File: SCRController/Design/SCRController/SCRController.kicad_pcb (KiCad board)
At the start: 2 copper layers, 76.9 x 73 mm, 43 parts, among them J1 VALT, J2 SAL_TRIAC, Q1 2N2907A, Q2 2N2222A, Q3 2N2222A, Q4 2N2907A, U1 TL084, U2 TL084, U3 LM7815_TO220, U4 LM7915_TO220, U5 MOC3011M

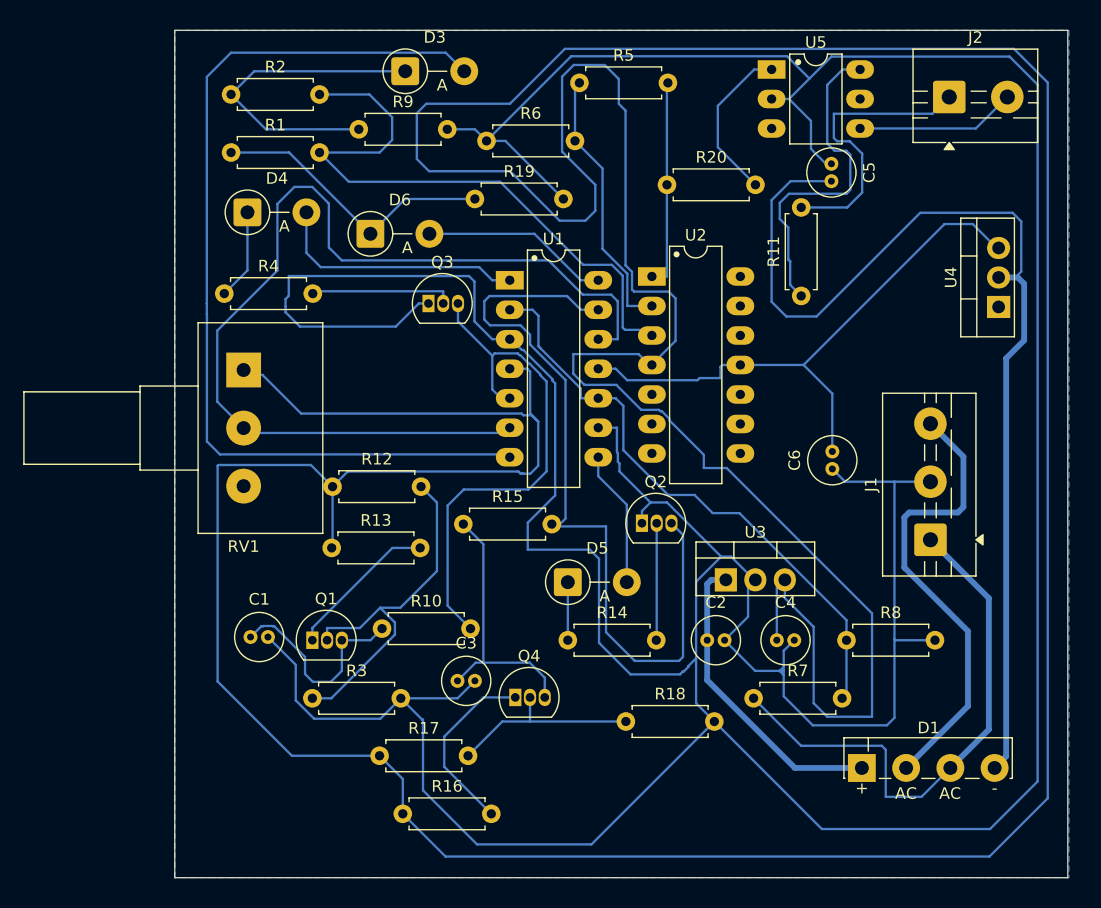
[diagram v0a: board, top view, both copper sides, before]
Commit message: rehecho
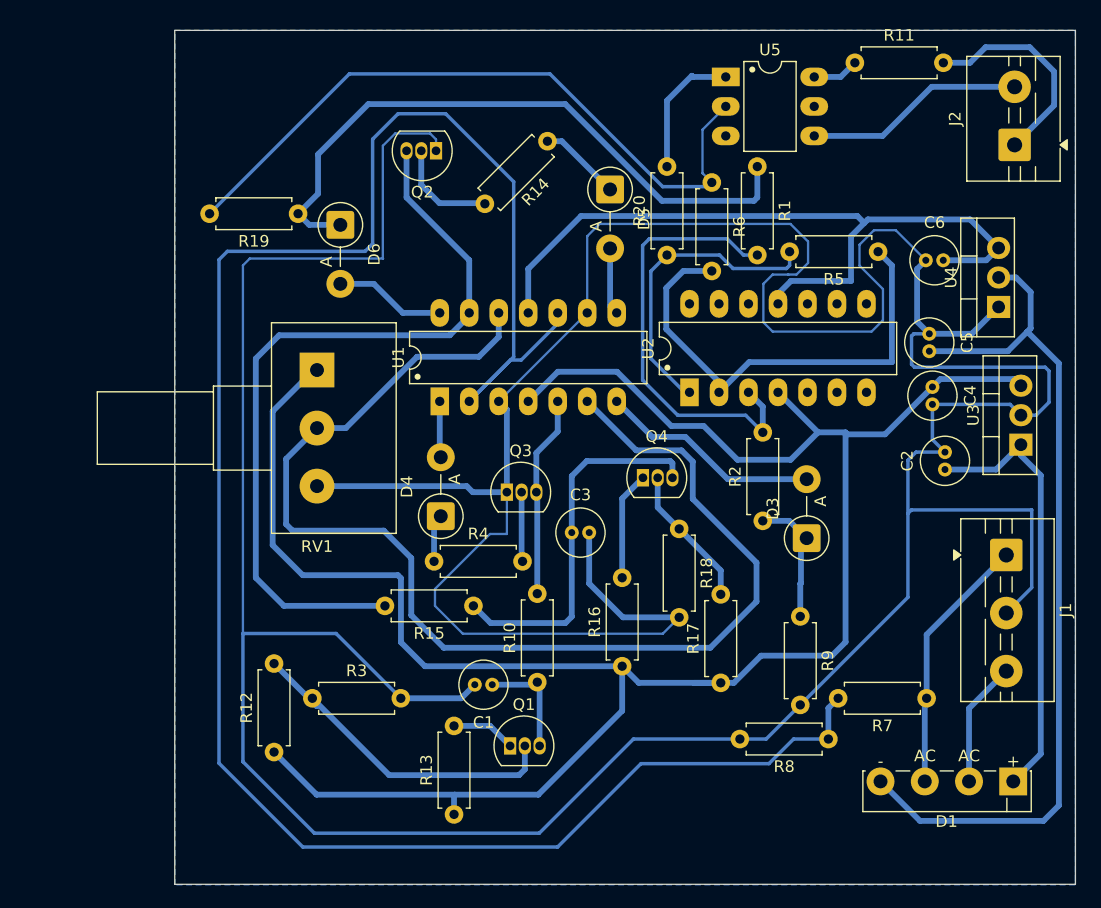
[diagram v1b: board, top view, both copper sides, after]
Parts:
- moved R2 58.7 mm to (80.5, 61.8), turned to 90 degrees
- moved R9 56.6 mm to (83.7, 70.0), turned to -90 degrees
- moved D3 53.0 mm to (84.3, 63.2), turned to 90 degrees
- moved R1 45.3 mm to (80.0, 31.2), turned to -90 degrees
- moved R14 43.0 mm to (61.9, 29.1), turned to -135 degrees
- moved Q2 36.7 mm to (52.3, 29.9), turned to 180 degrees
- moved D5 34.0 mm to (67.3, 33.2), turned to -90 degrees
- moved D4 31.0 mm to (52.8, 61.4), turned to 90 degrees
- moved R17 30.0 mm to (76.9, 75.7), turned to 90 degrees
- moved R5 29.5 mm to (90.4, 38.6), turned to 180 degrees
- moved R4 29.3 mm to (52.2, 65.2)
- moved U3 27.9 mm to (102.7, 55.2), turned to 90 degrees
- moved C4 25.6 mm to (95.1, 50.2), turned to -90 degrees
- moved R13 25.3 mm to (53.9, 87.0), turned to 90 degrees
- moved C2 25.2 mm to (96.2, 57.3), turned to 90 degrees
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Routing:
- net VCC: track 436.5 -> 190.9 mm
- net VSync: track 51.4 -> 176.6 mm
- net Net-(D3-A): track 81.7 -> 19.1 mm
- net Earth: track 420.4 -> 452.9 mm
- net A2: track 25.1 -> 55.7 mm
- net VA-: track 39.9 -> 10.8 mm
- net Net-(Q3-C): track 45.1 -> 17.4 mm
- net Net-(R11-Pad1): track 29.4 -> 4.01 mm
- net VA+: track 47.0 -> 22.4 mm
- net VCOMP: track 86.8 -> 105.9 mm
- net VDC-: track 93.7 -> 75.2 mm
- net Net-(U2A--): track 23.1 -> 41.4 mm
- net Net-(D4-A): track 22.0 -> 4.85 mm
- net A1: track 28.1 -> 11.4 mm
- net VEE: track 50.4 -> 65.9 mm
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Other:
- board size 76.9 x 73 mm -> 77.6 x 73.5 mm
